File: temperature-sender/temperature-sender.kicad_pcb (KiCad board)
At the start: 2 copper layers, 50 x 25 mm, 43 parts, among them IC1 ATTINY2313A-S, K1 SERVO, P1 CONN_01X02, P2 CONN_01X02, P3 CONN_01X02, P6 ISP, P7 CONN_01X03, P8 CONN_01X03, SW1 SW_PUSH, SW2 SW_PUSH, U1 MCP1700T-3302E/TT, U2 TMP102, U3 78L09, U4 HT7550-1

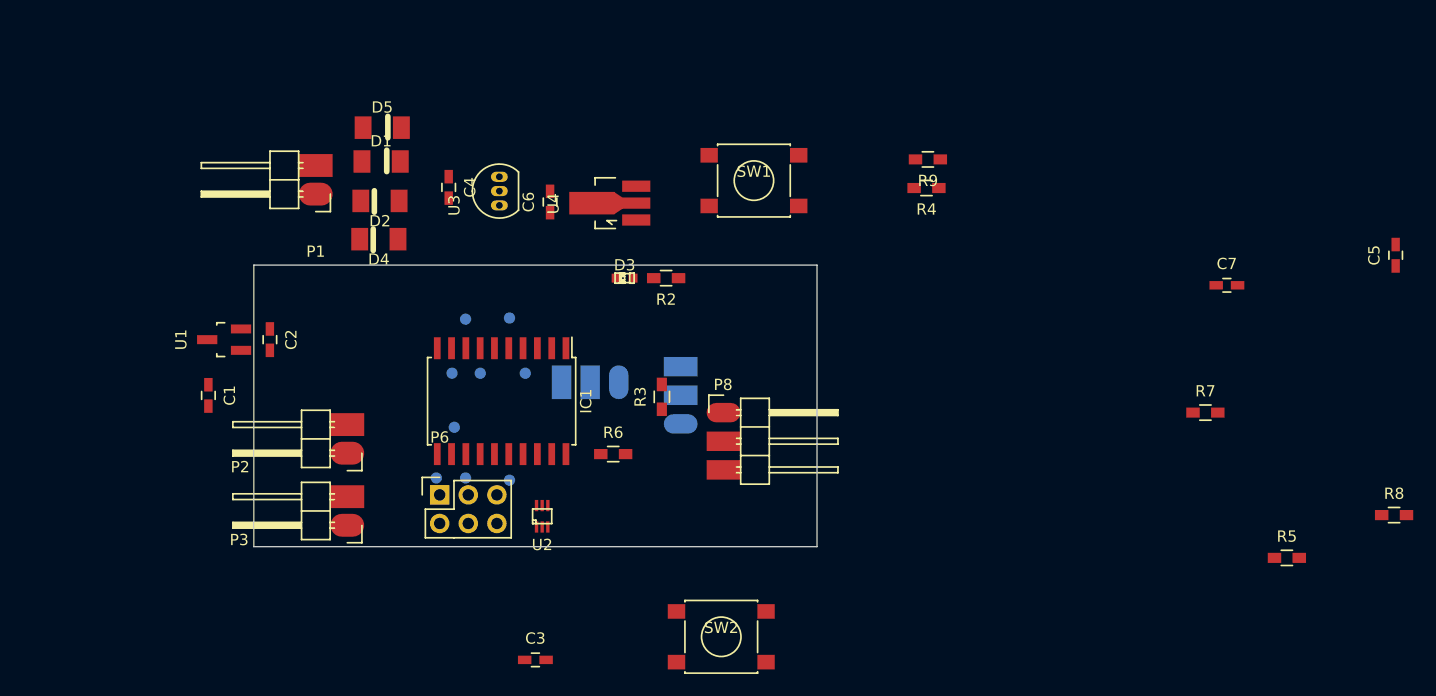
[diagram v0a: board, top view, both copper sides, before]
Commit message: Some more changes, slowly getting there
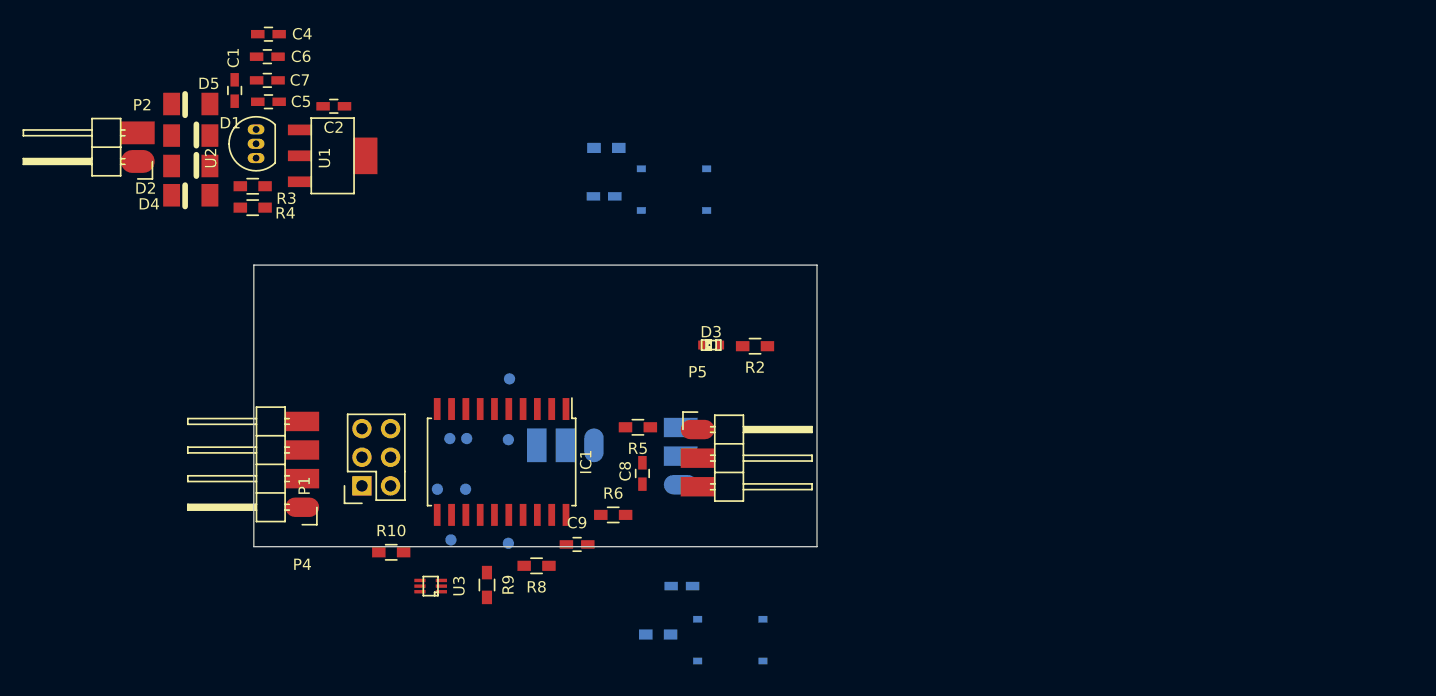
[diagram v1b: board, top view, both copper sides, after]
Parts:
- removed P6: ISP, Socket_Strips:Socket_Strip_Straight_2x03
- removed P7, P8: CONN_01X03, kicad-footprints:Pin_Header_Angled_SMD_1x03
- removed TP_PB0, TP_PB4, TP_PD4, TP_PD5, TP_PD6: TEST_POINT, kicad-footprints:TP_1mm
- removed U4: HT7550-1, Housings_SOT-89:SOT89-3_Housing_Handsoldering
- added C10: 0.1uF, Capacitors_SMD:C_0603_HandSoldering, B.Cu at (143.0, 148.5)
- added C8: 10uF, Capacitors_SMD:C_0603_HandSoldering, F.Cu at (139.5, 138.5)
- added C9: 10uF, Capacitors_SMD:C_0603_HandSoldering, F.Cu at (133.7, 144.8)
- added P4: CONN_01X04, kicad-footprints:Pin_Header_Angled_SMD_1x04, F.Cu at (109.3, 141.5)
- added P5: CONN_01X03, kicad-footprints:Pin_Header_Angled_SMD_1x03, F.Cu at (144.4, 134.6)
- added R1: 47k, Resistors_SMD:R_0603_HandSoldering, B.Cu at (136.3, 109.6)
- added R10: 5k, Resistors_SMD:R_0603_HandSoldering, F.Cu at (117.2, 145.5)
- added TP_PB2: TEST_POINT, kicad-footprints:TP_1mm, B.Cu at (123.7, 139.9)
- added TP_PB3: TEST_POINT, kicad-footprints:TP_1mm, B.Cu at (127.5, 144.7)
- added TP_PD1: TEST_POINT, kicad-footprints:TP_1mm, B.Cu at (123.8, 135.4)
- added TP_PD2: TEST_POINT, kicad-footprints:TP_1mm, B.Cu at (122.3, 135.4)
- C1: value 10uF -> 1uF
- C2, C4: value 1uF -> 10uF
- C3: value C -> 0.1uF; moved to B.Cu
- C5, C7: value 0.1uF -> 10uF
- P1: value CONN_01X02 -> ISP; footprint kicad-footprints:Pin_Header_Angled_SMD_1x02 -> Socket_Strips:Socket_Strip_Straight_2x03
- P3: value CONN_01X02 -> CONN_01X03; footprint kicad-footprints:Pin_Header_Angled_SMD_1x02 -> kicad-footprints:Pin_Header_Angled_SMD_1x03; moved to B.Cu
- R3: value 5k -> 240R
- R4: value 47R -> 1k5
- R5, R6: value 47k -> 47R
- R7: value 5k -> 47k; moved to B.Cu
- R9: value 47R -> 5k
- SW1, SW2: footprint Buttons_Switches_SMD:SW_SPST_PTS645 -> kicad-footprints:4x4x1.5mm_Tactile_Push_Button_SMD; moved to B.Cu
- U1: value MCP1700T-3302E/TT -> AMS1117; footprint Housings_SOT-23_SOT-143_TSOT-6:SOT-23_Handsoldering -> kicad-footprints:SOT-223
- U2: value TMP102 -> LM317L; footprint kicad-footprints:SOT563 -> Housings_TO-92:TO-92_Inline_Narrow_Oval
- U3: value 78L09 -> TMP102; footprint Housings_TO-92:TO-92_Inline_Narrow_Oval -> kicad-footprints:SOT563
- moved C5 101.0 mm to (106.3, 105.5), turned to 0 degrees
- moved C7 87.1 mm to (106.2, 103.6)
- moved R8 76.3 mm to (130.1, 146.7), turned to 180 degrees
- moved R4 59.8 mm to (104.9, 114.9)
- moved R5 58.8 mm to (139.1, 134.4), turned to 180 degrees
- moved R9 54.4 mm to (125.7, 148.4), turned to 270 degrees
- moved R7 52.4 mm to (140.9, 152.8)
- moved C3 41.6 mm to (136.1, 113.9)
- moved R3 40.9 mm to (104.9, 113.0), turned to 0 degrees
- moved U2 40.7 mm to (105.2, 110.5), turned to 90 degrees
- moved U3 34.3 mm to (120.7, 148.5)
- moved P2 31.9 mm to (94.7, 110.8)
- moved C6 28.2 mm to (106.2, 101.5), turned to 0 degrees
- moved C1 27.2 mm to (103.3, 104.5)
- moved P1 26.2 mm to (114.6, 139.6), turned to 90 degrees
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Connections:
- C1 pad 1: +5V -> /Vin_rec
- C3 pad 1: /SERVO_PWR -> GND
- C3 pad 2: GND -> /SW
- C4 pad 1: Net-(C4-Pad1) -> /9v
- C5 pad 1: /RESET -> /9v
- C6 pad 1: +9V -> /9v
- C7 pad 1: GND -> /9v
- C7 pad 2: Net-(C7-Pad2) -> GND
- D1 pad 1: Net-(C4-Pad1) -> /Vin_rec
- D1 pad 2: Net-(D1-Pad2) -> /Vin1
- D2 pad 1: Net-(D2-Pad1) -> /Vin_rec
- D2 pad 2: GND -> /Vin2
- D4 pad 1: Net-(D1-Pad2) -> /Vin2
- D5 pad 1: Net-(C4-Pad1) -> /Vin1
- D5 pad 2: Net-(D2-Pad1) -> GND
- IC1 pad 7: Net-(IC1-Pad7) -> /SW
- K1 pad 3: Net-(K1-Pad3) -> /SERVO_SIG
- P1 pad 1: Net-(D2-Pad1) -> /MISO
- P1 pad 2: Net-(D1-Pad2) -> +3V3
- P2 pad 1: /SDA/MOSI -> /Vin2
- P2 pad 2: /SCL -> /Vin1
- P3 pad 2: +3V3 -> /TX
- R3 pad 1: /ALERT -> /Vadj
- R3 pad 2: +3V3 -> /9v
- R4 pad 1: Net-(K1-Pad3) -> GND
- R4 pad 2: /SERVO1 -> /Vadj
- R5 pad 1: +3V3 -> /SERVO_SIG
- R5 pad 2: /RESET -> /SERVO1
- R6 pad 1: +3V3 -> /SERVO_PWR
- R6 pad 2: Net-(C7-Pad2) -> +3V3
- R7 pad 2: /SCL -> /RESET
- R9 pad 1: /SERVO_PWR -> +3V3
- R9 pad 2: +3V3 -> /SCL
- SW1 pad 1: GND -> /SW
- SW1 pad 2: /RESET -> GND
- SW2 pad 1: Net-(C7-Pad2) -> GND
- SW2 pad 2: GND -> /RESET
- TP_PB1 pad 1: Net-(IC1-Pad13) -> Net-(IC1-Pad12)
- TP_PD3 pad 1: Net-(IC1-Pad7) -> Net-(IC1-Pad11)
- TP_XTAL1 pad 1: Net-(IC1-Pad5) -> Net-(IC1-Pad4)
- TP_XTAL2 pad 1: Net-(IC1-Pad4) -> Net-(IC1-Pad5)
- U1 pad 3: +5V -> /9v
- U2 pad 1: /SCL -> /Vadj
- U2 pad 2: GND -> /9v
- U2 pad 3: /ALERT -> /Vin_rec
- U3 pad 1: +9V -> /SCL
- U3 pad 3: Net-(C4-Pad1) -> /ALERT
